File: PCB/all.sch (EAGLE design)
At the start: 120 parts, among them J1 ISP Programmer, J2 LIPO-BATTERY-CONNECTOR, J3 Qi coil, J4 Qi coil, J5 Qi coil, J6 Qi coil, J7 UART, J8 BL-HP20AUW2C, Q1 NPN, Q2 NPN, U1 ATTINY1634MLF20, U2 LM3671, U3 MPU-6050-1, U4 BQ51013B_RHL_20, U5 MCP73831, U6 CAT4139, U7 BQ51013B_RHL_20, U8 BQ51013B_RHL_20, U9 BQ51013B_RHL_20

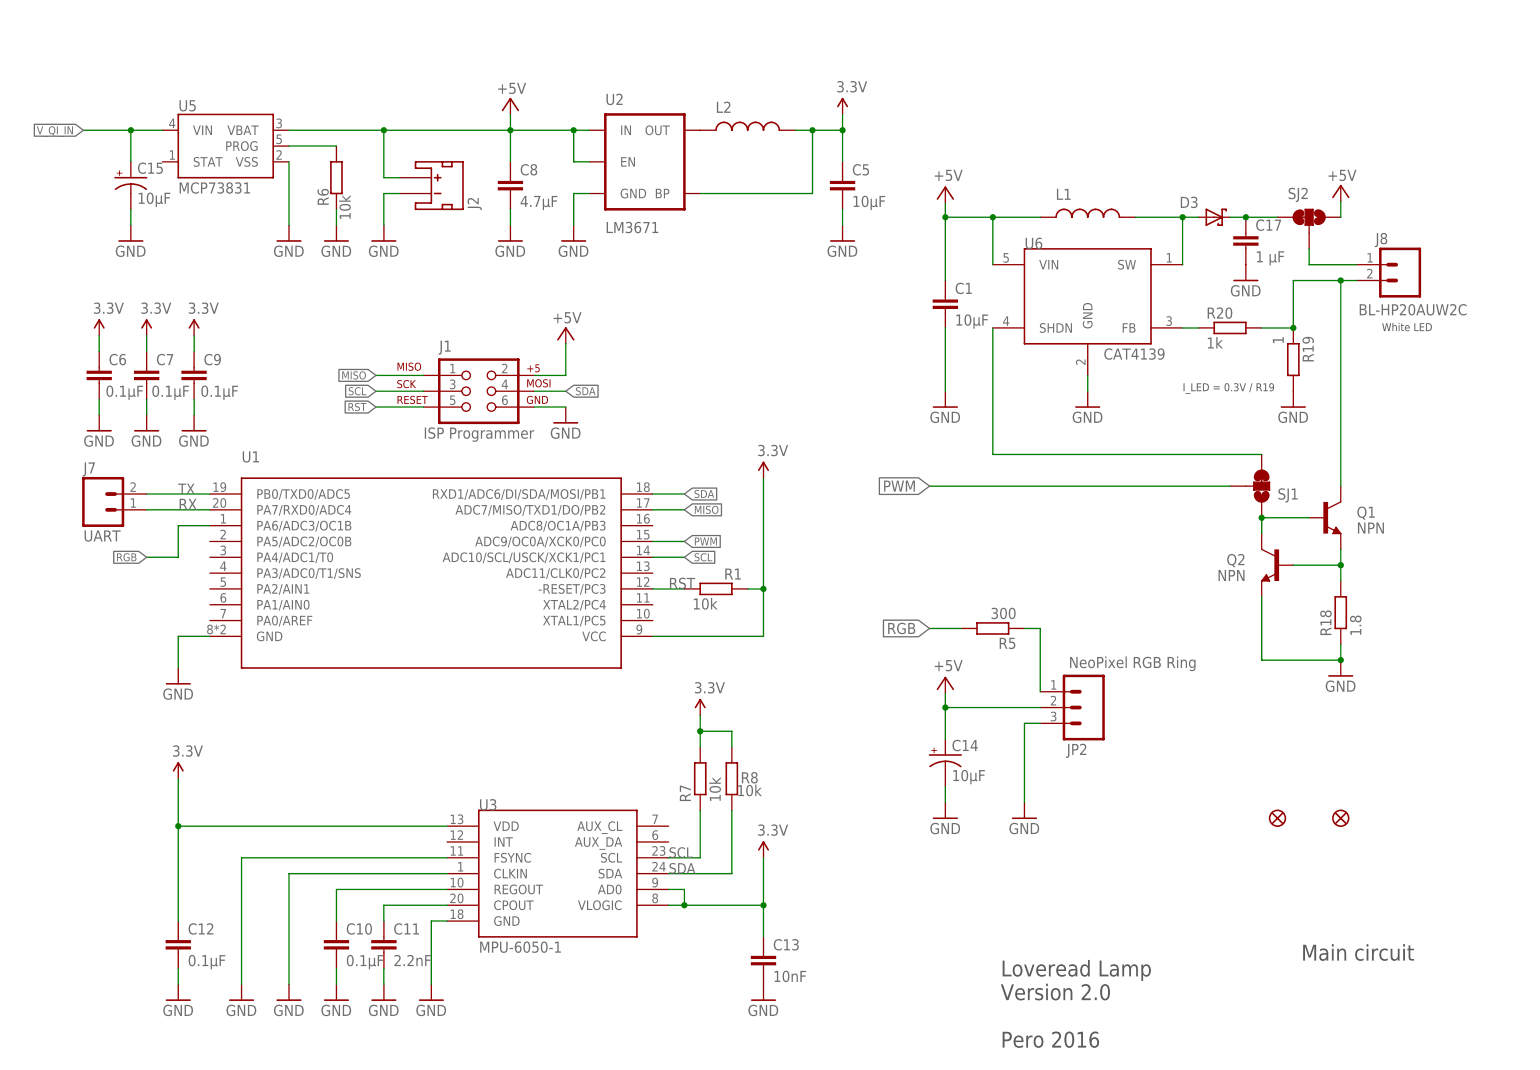
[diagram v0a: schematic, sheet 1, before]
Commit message: going back to 32u4
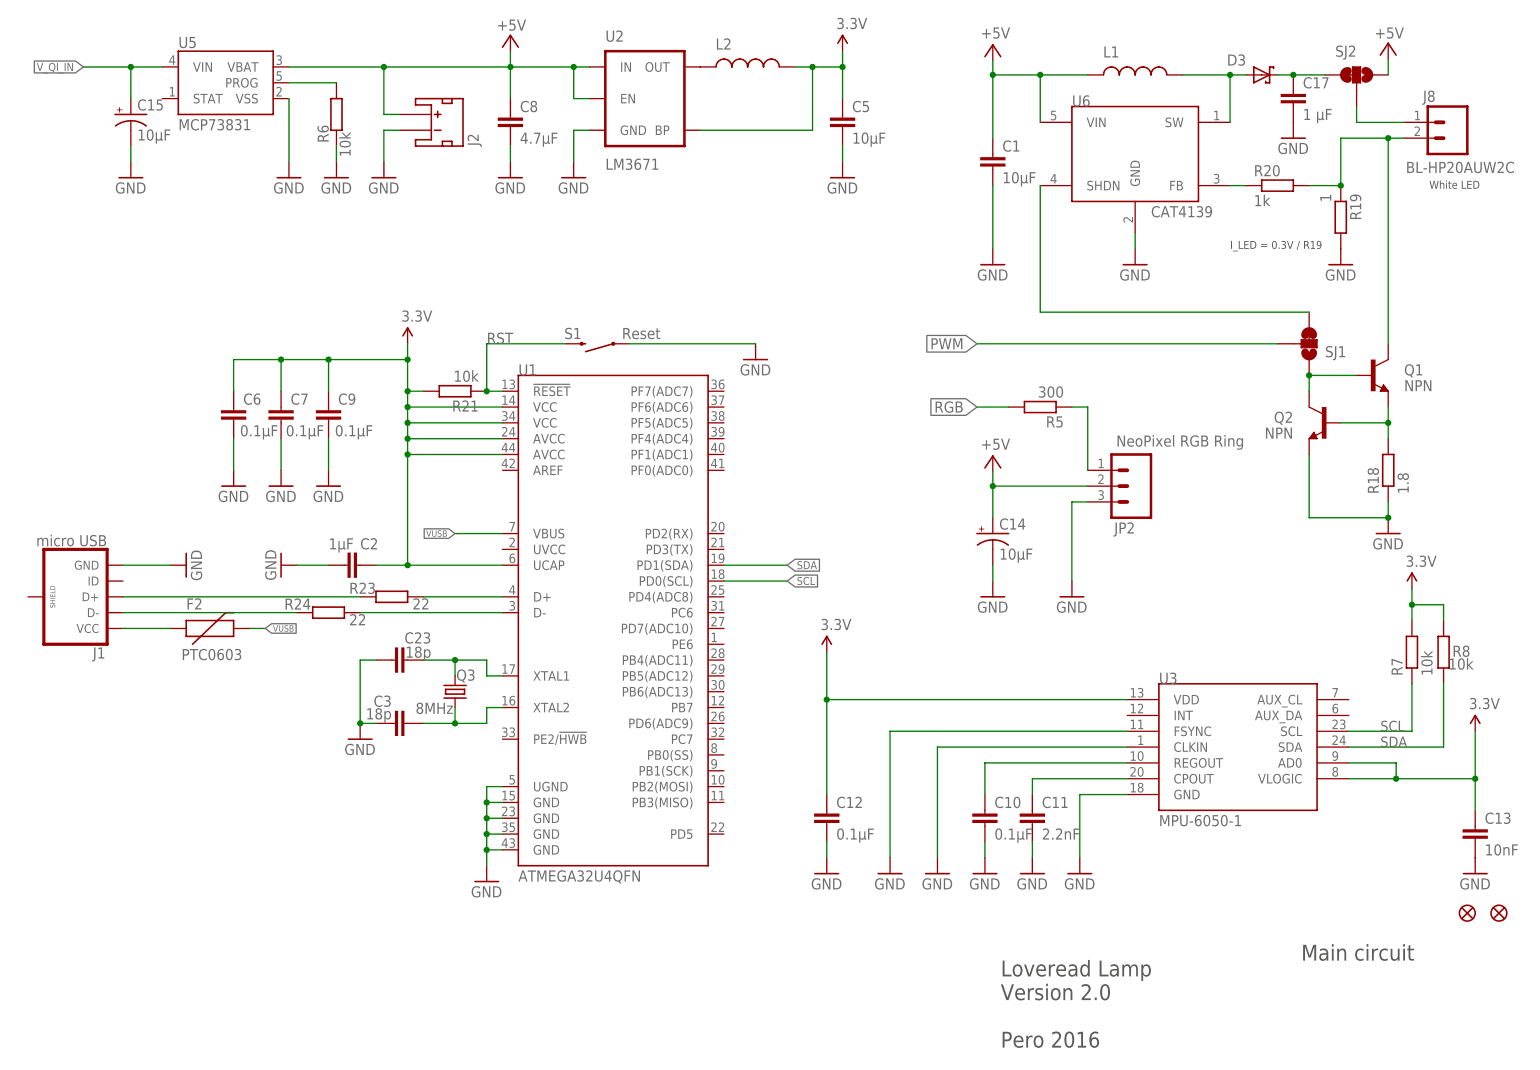
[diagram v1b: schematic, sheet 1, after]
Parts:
- removed J7: UART, SparkFun-Connectors:M02PTH
- removed R1: 10k, rcl:R-EU_R0603
- added C2: 1µF, rcl:C-EUC0603
- added C23, C3: 18p, rcl:C-EUC0603
- added F2: PTC0603, SparkFun-PowerIC:PTC0603
- added Q3: 8MHz, pero_library:QUARTZ-CRYSTAL-8MHZQC6CB8.00000F18B23R
- added R21: 10k, rcl:R-EU_R0603
- added R23, R24: 22, rcl:R-EU_R0603
- added S1: Reset, pero_library:SWITCH-BUTTON-SKSGAAE010
- J1: value ISP Programmer -> micro USB; device SparkFun:AVR_SPI_PRG_6PTH -> SparkFun-Connectors:USB_MICROB_PLUGCONN-11752
- L2: value 22uH -> 2.2uH
- U1: value ATTINY1634MLF20 -> ATMEGA32U4QFN; device attiny1634:ATTINY1634MLF20 -> SparkFun-DigitalIC:ATMEGA32U4QFN
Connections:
- removed net MISO: J1.1, U1.ADC7/MISO/TXD1/DO/PB2
- removed net RX: J7.1, U1.PA7/RXD0/ADC4
- removed net TX: J7.2, U1.PB0/TXD0/ADC5
- new net N$71: C23.2, Q3.2, U1.XTAL1
- new net N$72: C3.2, Q3.1, U1.XTAL2
- new net N$73: F2.1, J1.VCC
- new net N$74: J1.D+, R23.1
- new net N$78: J1.D-, R24.1
- new net N$80: R23.2, U1.D+
- new net N$81: R24.2, U1.D-
- new net VUSB: F2.2, U1.VBUS
- net +5V: no longer J1.2
- net 3.3V: now also C2.1, R21.2, U1.AVCC@24, U1.AVCC@44, U1.UCAP, U1.VCC@14, U1.VCC@34; no longer R1.2, U1.VCC
- net GND: now also C2.2, C23.1, C3.1, J1.GND, S1.1, U1.GND@15, U1.GND@23, U1.GND@35, U1.GND@43, U1.UGND; no longer J1.6, U1.GND
- net PWM: no longer U1.ADC9/OC0A/XCK0/PC0
- net RGB: no longer U1.PA6/ADC3/OC1B
- net RST: now also R21.1, S1.2, U1.!RESET; no longer J1.5, R1.1, U1.-RESET/PC3
- net SCL: now also U1.PD0(SCL); no longer J1.3, U1.ADC10/SCL/USCK/XCK1/PC1
- net SDA: now also U1.PD1(SDA); no longer J1.4, U1.RXD1/ADC6/DI/SDA/MOSI/PB1
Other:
- moved on the sheet: C1, C10, C11, C12, C13, C14, C15, C17, C5, C6, C7, C8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
